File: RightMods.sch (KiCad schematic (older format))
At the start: 13 parts

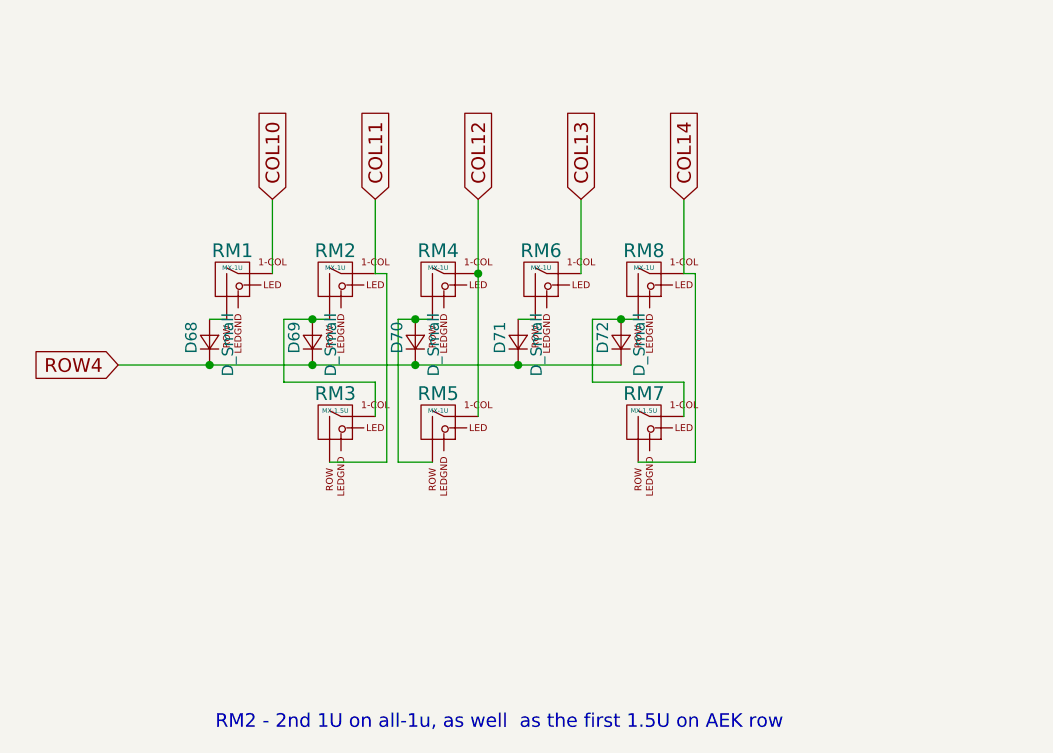
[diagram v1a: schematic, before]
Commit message: Update right mods
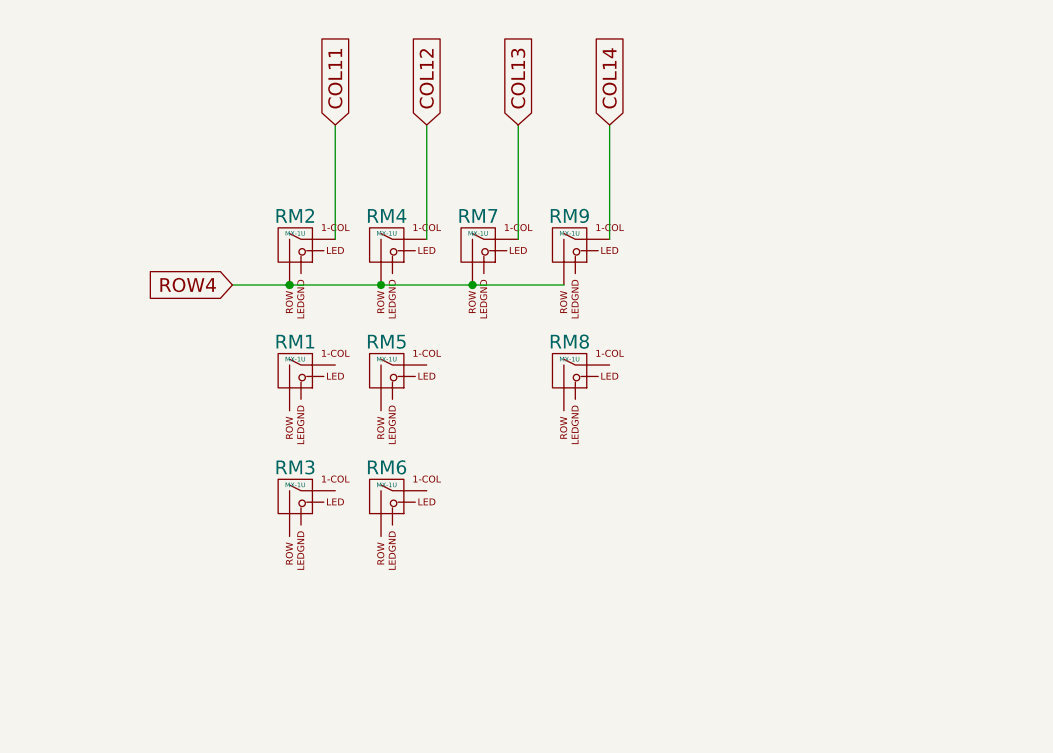
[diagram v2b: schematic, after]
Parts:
- removed D68, D69, D70, D71, D72: D_Small, Diodes_SMD:D_SOD-123, symbol D_Small
- added RM9: MX-1U, symbol MX-1U
- RM1, RM2, RM4, RM5, RM6, RM8: footprint MX_Alps_Hybrid:MX-1U-NoLED -> (none)
- RM3, RM7: value MX-1.5U -> MX-1U; footprint MX_Alps_Hybrid:MX-1.5U-NoLED -> (none)
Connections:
- net COL11: no longer RM3.2 (ROW)
- net COL12: no longer RM5.1 (COL)
- net COL13: now also RM7.1 (COL); no longer RM6.1 (COL)
- net COL14: now also RM9.1 (COL); no longer RM7.2 (ROW), RM8.1 (COL)
- net ROW4: now also RM2.2 (ROW), RM4.2 (ROW), RM7.2 (ROW), RM9.2 (ROW)
- net at RM3.1 (COL): no longer RM2.2 (ROW)
- net at RM5.2 (ROW): no longer RM4.2 (ROW)
- net at RM8.2 (ROW): no longer RM7.1 (COL)
- net COL10: no longer names the net of RM1.1 (COL)
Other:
- note removed: "RM2 - 2nd 1U on all-1u, as well as the first 1.5U on AEK row"
